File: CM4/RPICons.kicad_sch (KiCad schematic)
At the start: 8 parts, among them U1 Compute_Module_4_Connectors

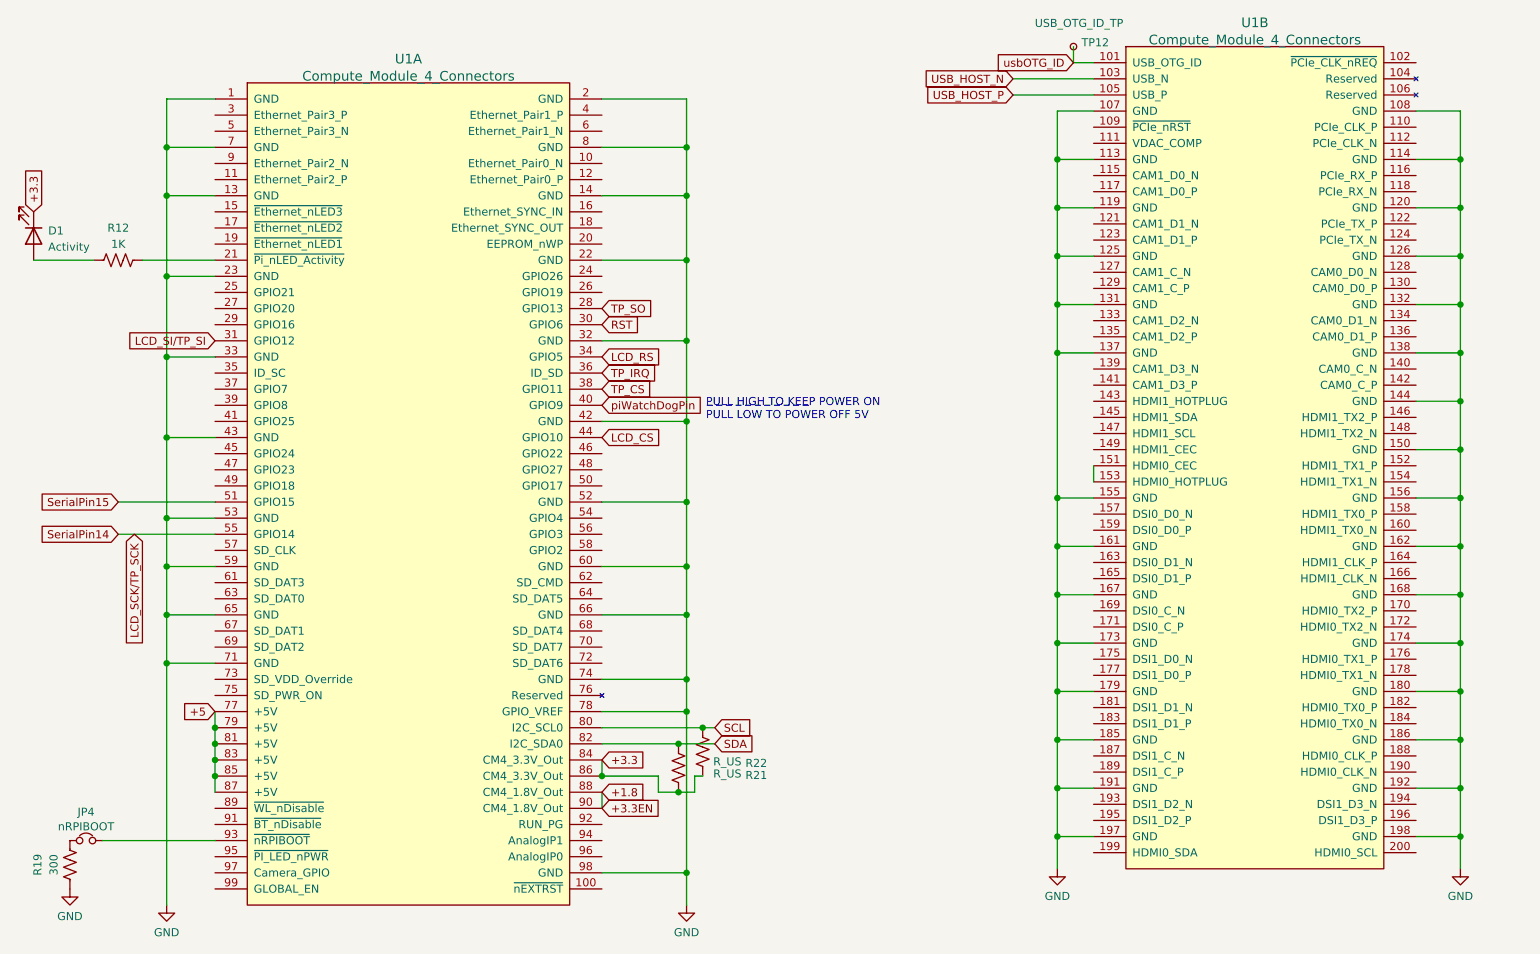
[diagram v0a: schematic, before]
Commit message: PrepedHDMIConnections
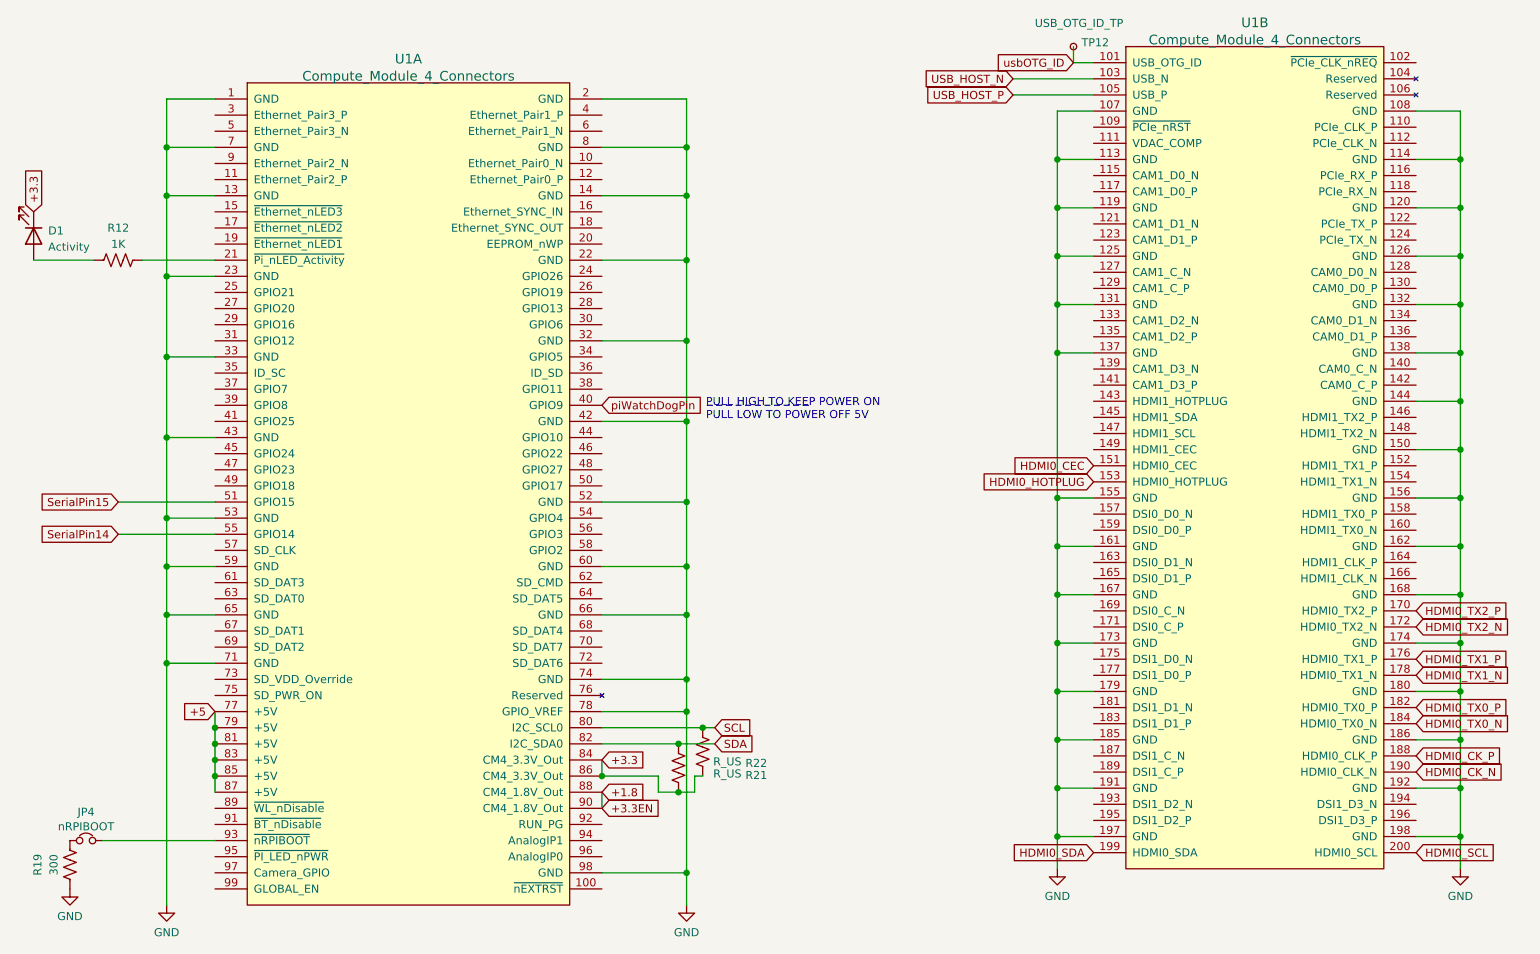
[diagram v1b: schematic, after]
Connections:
- net HDMI0_CEC: now reaches U1.151 (HDMI0_CEC)
- net HDMI0_CEC: no longer U1.153 (HDMI0_HOTPLUG)
- net HDMI0_TX2_P: now reaches U1.170 (HDMI0_TX2_P)
- net HDMI0_TX2_N: now reaches U1.172 (HDMI0_TX2_N)
- net HDMI0_TX1_P: now reaches U1.176 (HDMI0_TX1_P)
- net HDMI0_TX1_N: now reaches U1.178 (HDMI0_TX1_N)
- net HDMI0_TX0_P: now reaches U1.182 (HDMI0_TX0_P)
- net HDMI0_TX0_N: now reaches U1.184 (HDMI0_TX0_N)
- net HDMI0_CK_P: now reaches U1.188 (HDMI0_CLK_P)
- net HDMI0_CK_N: now reaches U1.190 (HDMI0_CLK_N)
- net HDMI0_SDA: now reaches U1.199 (HDMI0_SDA)
- net HDMI0_SCL: now reaches U1.200 (HDMI0_SCL)
- net LCD_CS: no longer names the net of U1.44 (GPIO10)
- net LCD_RS: no longer names the net of U1.34 (GPIO5)
- net LCD_SCK/TP_SCK renamed SerialPin14
- net LCD_SI/TP_SI: no longer names the net of U1.31 (GPIO12)
- net RST: no longer names the net of U1.30 (GPIO6)
- net TP_CS: no longer names the net of U1.38 (GPIO11)
- net TP_IRQ: no longer names the net of U1.36 (ID_SD)
- net TP_SO: no longer names the net of U1.28 (GPIO13)
- new net HDMI0_HOTPLUG: U1.153 (HDMI0_HOTPLUG)
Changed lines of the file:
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@@
-    (stroke (width 0) (type solid) (color 0 0 0 0))
-  )
-  (wire (pts (xy 189.865 90.805) (xy 189.865 93.345))
     (stroke (width 0) (type solid) (color 0 0 0 0))
   )
@@
     )
   )
-  (global_label "LCD_SCK{slash}TP_SCK" (shape input) (at 38.735 101.6 270)
-    (effects (font (size 1.27 1.27)) (justify right))
-    (property "Intersheet References" "${INTERSHEET_REFS}" (id 0) (at 38.6556 120.5836 90)
-      (effects (font (size 1.27 1.27)) (justify right) hide)
-    )
-  )
-  (global_label "LCD_SI{slash}TP_SI" (shape input) (at 51.435 71.12 180)
-    (effects (font (size 1.27 1.27)) (justify right))
-    (property "Intersheet References" "${INTERSHEET_REFS}" (id 0) (at 36.3219 71.0406 0)
-      (effects (font (size 1.27 1.27)) (justify right) hide)
-    )
-  )
   (global_label "+5" (shape input) (at 51.435 129.54 180)
     (effects (font (size 1.27 1.27)) (justify right))
@@
     )
   )
-  (global_label "TP_SO" (shape input) (at 112.395 66.04 0)
-    (effects (font (size 1.27 1.27)) (justify left))
-    (property "Intersheet References" "${INTERSHEET_REFS}" (id 0) (at 120.5533 65.9606 0)
-      (effects (font (size 1.27 1.27)) (justify left) hide)
-    )
-  )
-  (global_label "RST" (shape input) (at 112.395 68.58 0)
-    (effects (font (size 1.27 1.27)) (justify left))
-    (property "Intersheet References" "${INTERSHEET_REFS}" (id 0) (at 118.2552 68.5006 0)
-      (effects (font (size 1.27 1.27)) (justify left) hide)
-    )
-  )
-  (global_label "LCD_RS" (shape input) (at 112.395 73.66 0)
-    (effects (font (size 1.27 1.27)) (justify left))
-    (property "Intersheet References" "${INTERSHEET_REFS}" (id 0) (at 121.8233 73.5806 0)
-      (effects (font (size 1.27 1.27)) (justify left) hide)
-    )
-  )
-  (global_label "TP_IRQ" (shape input) (at 112.395 76.2 0)
-    (effects (font (size 1.27 1.27)) (justify left))
-    (property "Intersheet References" "${INTERSHEET_REFS}" (id 0) (at 121.2186 76.1206 0)
-      (effects (font (size 1.27 1.27)) (justify left) hide)
-    )
-  )
-  (global_label "TP_CS" (shape input) (at 112.395 78.74 0)
-    (effects (font (size 1.27 1.27)) (justify left))
-    (property "Intersheet References" "${INTERSHEET_REFS}" (id 0) (at 120.4929 78.6606 0)
-      (effects (font (size 1.27 1.27)) (justify left) hide)
-    )
-  )
   (global_label "piWatchDogPin" (shape input) (at 112.395 81.28 0)
     (effects (font (size 1.27 1.27)) (justify left))
@@
     )
   )
-  (global_label "LCD_CS" (shape input) (at 112.395 86.36 0)
-    (effects (font (size 1.27 1.27)) (justify left))
-    (property "Intersheet References" "${INTERSHEET_REFS}" (id 0) (at 121.8233 86.2806 0)
-      (effects (font (size 1.27 1.27)) (justify left) hide)
-    )
-  )
   (global_label "+3.3" (shape input) (at 112.395 137.16 0)
     (effects (font (size 1.27 1.27)) (justify left))
@@
     )
   )
+  (global_label "HDMI0_CEC" (shape input) (at 189.865 90.805 180)
+    (effects (font (size 1.27 1.27)) (justify right))
+    (property "Intersheet References" "${INTERSHEET_REFS}" (id 0) (at 176.929 90.7256 0)
+      (effects (font (size 1.27 1.27)) (justify right) hide)
+    )
+  )
+  (global_label "HDMI0_HOTPLUG" (shape input) (at 189.865 93.345 180)
+    (effects (font (size 1.27 1.27)) (justify right))
+    (property "Intersheet References" "${INTERSHEET_REFS}" (id 0) (at 172.0909 93.2656 0)
+      (effects (font (size 1.27 1.27)) (justify right) hide)
+    )
+  )
+  (global_label "HDMI0_SDA" (shape input) (at 189.865 151.765 180)
+    (effects (font (size 1.27 1.27)) (justify right))
+    (property "Intersheet References" "${INTERSHEET_REFS}" (id 0) (at 177.05 151.6856 0)
+      (effects (font (size 1.27 1.27)) (justify right) hide)
+    )
+  )
+  (global_label "HDMI0_TX2_P" (shape input) (at 240.665 113.665 0)
+    (effects (font (size 1.27 1.27)) (justify left))
+    (property "Intersheet References" "${INTERSHEET_REFS}" (id 0) (at 255.5362 113.5856 0)
+      (effects (font (size 1.27 1.27)) (justify left) hide)
+    )
+  )
+  (global_label "HDMI0_TX2_N" (shape input) (at 240.665 116.205 0)
+    (effects (font (size 1.27 1.27)) (justify left))
+    (property "Intersheet References" "${INTERSHEET_REFS}" (id 0) (at 255.5967 116.1256 0)
+      (effects (font (size 1.27 1.27)) (justify left) hide)
+    )
+  )
+  (global_label "HDMI0_TX1_P" (shape input) (at 240.665 121.285 0)
+    (effects (font (size 1.27 1.27)) (justify left))
+    (property "Intersheet References" "${INTERSHEET_REFS}" (id 0) (at 255.5362 121.2056 0)
+      (effects (font (size 1.27 1.27)) (justify left) hide)
+    )
+  )
+  (global_label "HDMI0_TX1_N" (shape input) (at 240.665 123.825 0)
+    (effects (font (size 1.27 1.27)) (justify left))
+    (property "Intersheet References" "${INTERSHEET_REFS}" (id 0) (at 255.5967 123.7456 0)
+      (effects (font (size 1.27 1.27)) (justify left) hide)
+    )
+  )
+  (global_label "HDMI0_TX0_P" (shape input) (at 240.665 128.905 0)
+    (effects (font (size 1.27 1.27)) (justify left))
+    (property "Intersheet References" "${INTERSHEET_REFS}" (id 0) (at 255.5362 128.8256 0)
+      (effects (font (size 1.27 1.27)) (justify left) hide)
+    )
+  )
+  (global_label "HDMI0_TX0_N" (shape input) (at 240.665 131.445 0)
+    (effects (font (size 1.27 1.27)) (justify left))
+    (property "Intersheet References" "${INTERSHEET_REFS}" (id 0) (at 255.5967 131.3656 0)
+      (effects (font (size 1.27 1.27)) (justify left) hide)
+    )
+  )
+  (global_label "HDMI0_CK_P" (shape input) (at 240.665 136.525 0)
+    (effects (font (size 1.27 1.27)) (justify left))
+    (property "Intersheet References" "${INTERSHEET_REFS}" (id 0) (at 254.6895 136.4456 0)
+      (effects (font (size 1.27 1.27)) (justify left) hide)
+    )
+  )
+  (global_label "HDMI0_CK_N" (shape input) (at 240.665 139.065 0)
+    (effects (font (size 1.27 1.27)) (justify left))
+    (property "Intersheet References" "${INTERSHEET_REFS}" (id 0) (at 254.75 138.9856 0)
+      (effects (font (size 1.27 1.27)) (justify left) hide)
+    )
+  )
+  (global_label "HDMI0_SCL" (shape input) (at 240.665 151.765 0)
+    (effects (font (size 1.27 1.27)) (justify left))
+    (property "Intersheet References" "${INTERSHEET_REFS}" (id 0) (at 253.4195 151.6856 0)
+      (effects (font (size 1.27 1.27)) (justify left) hide)
+    )
+  )

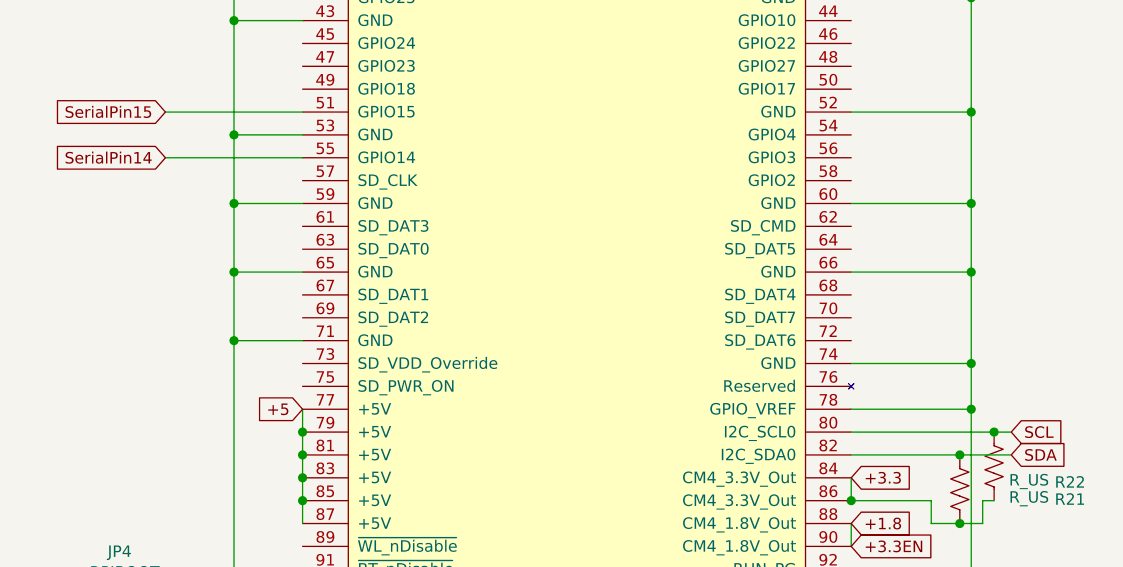
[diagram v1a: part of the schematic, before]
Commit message: added sdcard
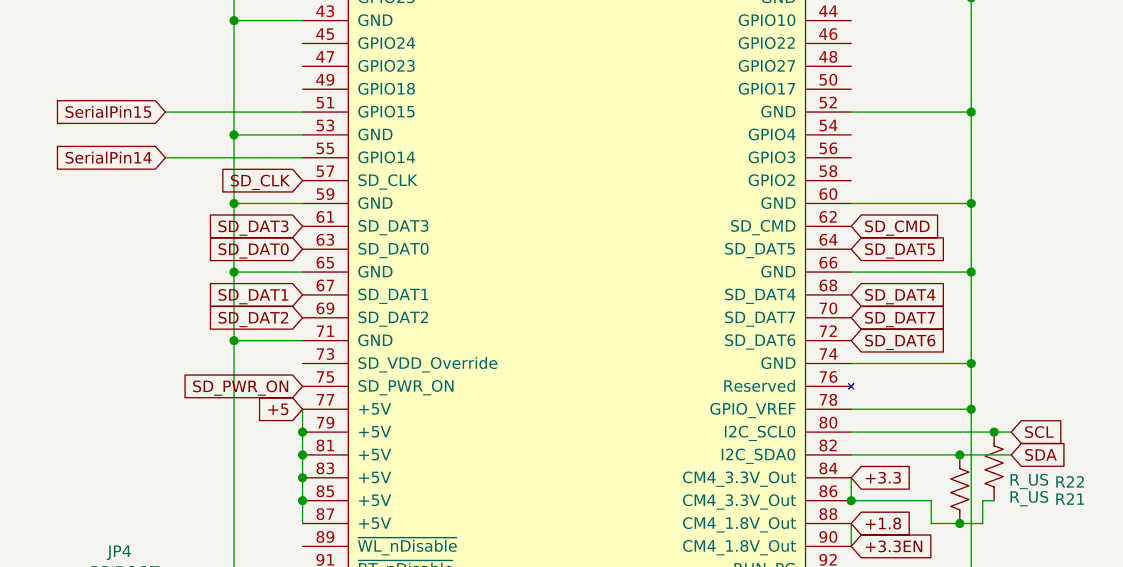
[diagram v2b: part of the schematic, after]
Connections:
- net SD_CLK: now reaches U1.57 (SD_CLK)
- net SD_DAT3: now reaches U1.61 (SD_DAT3)
- net SD_CMD: now reaches U1.62 (SD_CMD)
- net SD_DAT0: now reaches U1.63 (SD_DAT0)
- net SD_DAT5: now reaches U1.64 (SD_DAT5)
- net SD_DAT1: now reaches U1.67 (SD_DAT1)
- net SD_DAT4: now reaches U1.68 (SD_DAT4)
- net SD_DAT2: now reaches U1.69 (SD_DAT2)
- net SD_DAT7: now reaches U1.70 (SD_DAT7)
- net SD_DAT6: now reaches U1.72 (SD_DAT6)
- net SD_PWR_ON: now reaches U1.75 (SD_PWR_ON)
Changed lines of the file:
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@@
+    )
+  )
+  (global_label "SD_CLK" (shape input) (at 51.435 104.14 180)
+    (effects (font (size 1.27 1.27)) (justify right))
+    (property "Intersheet References" "${INTERSHEET_REFS}" (id 0) (at 42.0067 104.0606 0)
+      (effects (font (size 1.27 1.27)) (justify right) hide)
+    )
+  )
+  (global_label "SD_DAT3" (shape input) (at 51.435 109.22 180)
+    (effects (font (size 1.27 1.27)) (justify right))
+    (property "Intersheet References" "${INTERSHEET_REFS}" (id 0) (at 41.039 109.1406 0)
+      (effects (font (size 1.27 1.27)) (justify right) hide)
+    )
+  )
+  (global_label "SD_DAT0" (shape input) (at 51.435 111.76 180)
+    (effects (font (size 1.27 1.27)) (justify right))
+    (property "Intersheet References" "${INTERSHEET_REFS}" (id 0) (at 41.039 111.6806 0)
+      (effects (font (size 1.27 1.27)) (justify right) hide)
+    )
+  )
+  (global_label "SD_DAT1" (shape input) (at 51.435 116.84 180)
+    (effects (font (size 1.27 1.27)) (justify right))
+    (property "Intersheet References" "${INTERSHEET_REFS}" (id 0) (at 41.039 116.7606 0)
+      (effects (font (size 1.27 1.27)) (justify right) hide)
+    )
+  )
+  (global_label "SD_DAT2" (shape input) (at 51.435 119.38 180)
+    (effects (font (size 1.27 1.27)) (justify right))
+    (property "Intersheet References" "${INTERSHEET_REFS}" (id 0) (at 41.039 119.3006 0)
+      (effects (font (size 1.27 1.27)) (justify right) hide)
+    )
+  )
+  (global_label "SD_PWR_ON" (shape input) (at 51.435 127 180)
+    (effects (font (size 1.27 1.27)) (justify right))
+    (property "Intersheet References" "${INTERSHEET_REFS}" (id 0) (at 37.9548 126.9206 0)
+      (effects (font (size 1.27 1.27)) (justify right) hide)
     )
   )
@@
       (effects (font (size 1.27 1.27)) (justify left) hide)
     )
+  )
+  (global_label "SD_CMD" (shape input) (at 112.395 109.22 0)
+    (effects (font (size 1.27 1.27)) (justify left))
+    (property "Intersheet References" "${INTERSHEET_REFS}" (id 0) (at 122.2467 109.1406 0)
+      (effects (font (size 1.27 1.27)) (justify left) hide)
+    )
+  )
+  (global_label "SD_DAT5" (shape input) (at 112.395 111.76 0)
+    (effects (font (size 1.27 1.27)) (justify left))
+    (property "Intersheet References" "${INTERSHEET_REFS}" (id 0) (at 122.791 111.6806 0)
+      (effects (font (size 1.27 1.27)) (justify left) hide)
+    )
+  )
+  (global_label "SD_DAT4" (shape input) (at 112.395 116.84 0)
+    (effects (font (size 1.27 1.27)) (justify left))
+    (property "Intersheet References" "${INTERSHEET_REFS}" (id 0) (at 122.791 116.7606 0)
+      (effects (font (size 1.27 1.27)) (justify left) hide)
+    )
+  )
+  (global_label "SD_DAT7" (shape input) (at 112.395 119.38 0)
+    (effects (font (size 1.27 1.27)) (justify left))
+    (property "Intersheet References" "${INTERSHEET_REFS}" (id 0) (at 122.791 119.3006 0)
+      (effects (font (size 1.27 1.27)) (justify left) hide)
+    )
+  )
+  (global_label "SD_DAT6" (shape input) (at 112.395 121.92 0)
+    (effects (font (size 1.27 1.27)) (justify left))
+    (property "Intersheet References" "${INTERSHEET_REFS}" (id 0) (at 122.791 121.8406 0)
+      (effects (font (size 1.27 1.27)) (justify left) hide)
+    )
